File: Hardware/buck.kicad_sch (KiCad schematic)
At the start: 30 parts, among them Q301 SSM3K15AMFV,L3F, U301 SiC437AED-T1

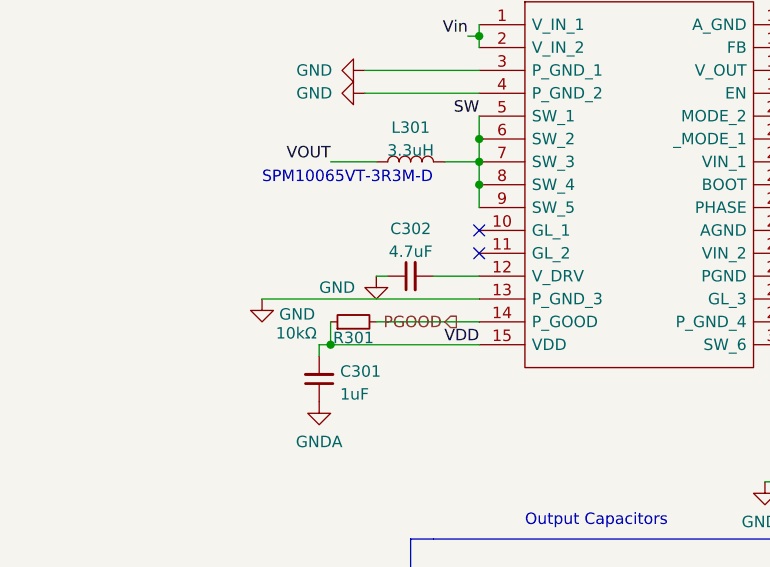
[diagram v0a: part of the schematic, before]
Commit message: prod files after final final change
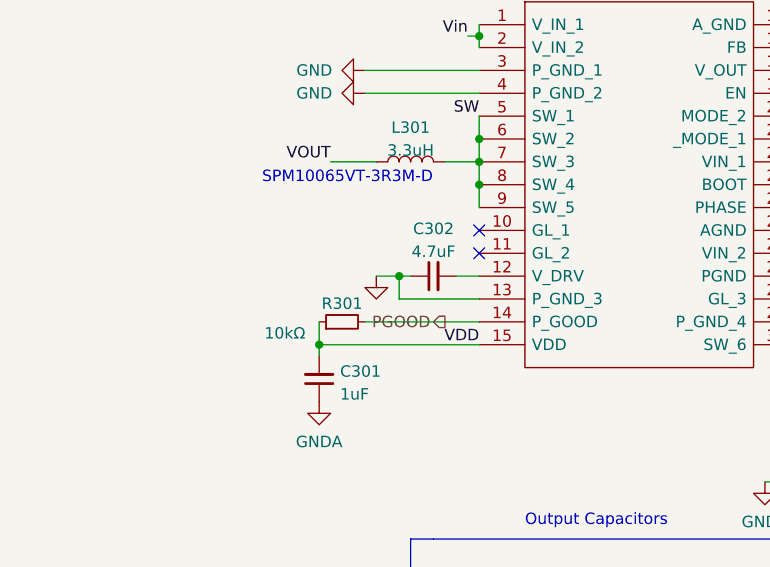
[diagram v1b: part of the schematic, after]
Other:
- moved on the sheet: C302, R301
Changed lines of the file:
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@@
 	)
 	(junction
-		(at 194.31 58.42)
+		(at 66.04 99.06)
 		(diameter 0)
 		(color 0 0 0 0)
 	)
 	(junction
-		(at 58.42 106.68)
+		(at 194.31 58.42)
 		(diameter 0)
 		(color 0 0 0 0)
@@
 	)
 	(junction
+		(at 57.15 106.68)
+		(diameter 0)
+		(color 0 0 0 0)
+	)
+	(junction
 		(at 208.28 77.47)
 		(diameter 0)
@@
 		)
 	)
+	(wire
+		(pts
+			(xy 66.04 99.06) (xy 66.04 101.6)
+		)
+		(stroke
+			(width 0)
+			(type default)
+		)
+	)
 	(polyline
 		(pts
@@
 	(wire
 		(pts
-			(xy 63.5 99.06) (xy 64.77 99.06)
-		)
-		(stroke
-			(width 0)
-			(type default)
-		)
-	)
-	(wire
-		(pts
-			(xy 58.42 104.14) (xy 58.42 106.68)
+			(xy 57.15 104.14) (xy 57.15 106.68)
 		)
 		(stroke
@@
 	(wire
 		(pts
-			(xy 86.36 140.97) (xy 91.44 140.97)
+			(xy 57.15 106.68) (xy 74.93 106.68)
 		)
 		(stroke
@@
 	(wire
 		(pts
-			(xy 58.42 106.68) (xy 57.15 106.68)
+			(xy 86.36 140.97) (xy 91.44 140.97)
 		)
 		(stroke
@@
 	(wire
 		(pts
-			(xy 63.5 104.14) (xy 74.93 104.14)
+			(xy 62.23 104.14) (xy 74.93 104.14)
 		)
 		(stroke
@@
 	(wire
 		(pts
+			(xy 66.04 101.6) (xy 74.93 101.6)
+		)
+		(stroke
+			(width 0)
+			(type default)
+		)
+	)
+	(wire
+		(pts
 			(xy 74.93 83.82) (xy 74.93 86.36)
 		)
@@
 	(wire
 		(pts
-			(xy 50.8 101.6) (xy 74.93 101.6)
+			(xy 63.5 99.06) (xy 66.04 99.06)
 		)
 		(stroke
@@
 	(wire
 		(pts
-			(xy 69.85 99.06) (xy 74.93 99.06)
+			(xy 72.39 99.06) (xy 74.93 99.06)
+		)
+		(stroke
+			(width 0)
+			(type default)
+		)
+	)
+	(wire
+		(pts
+			(xy 66.04 99.06) (xy 67.31 99.06)
 		)
 		(stroke
@@
 	(wire
 		(pts
-			(xy 58.42 106.68) (xy 74.93 106.68)
-		)
-		(stroke
-			(width 0)
-			(type default)
-		)
-	)
-	(wire
-		(pts
 			(xy 124.46 69.85) (xy 134.62 69.85)
 		)
@@
 	(hierarchical_label "PGOOD"
 		(shape output)
-		(at 72.39 104.14 180)
+		(at 71.12 104.14 180)
 		(effects
 			(font
@@
 	(symbol
 		(lib_id "Device:C_Small")
-		(at 67.31 99.06 90)
+		(at 69.85 99.06 90)
 		(unit 1)
 		(exclude_from_sim no)
@@
 		(fields_autoplaced yes)
 		(property "Reference" "C302"
-			(at 67.3163 93.7981 90)
+			(at 69.8563 93.7981 90)
 			(effects
 				(font
@@
 		)
 		(property "Value" "4.7uF"
-			(at 67.3163 96.335 90)
+			(at 69.8563 96.335 90)
 			(effects
 				(font
@@
 		)
 		(property "Footprint" "Capacitor_SMD:C_0402_1005Metric"
-			(at 67.31 99.06 0)
+			(at 69.85 99.06 0)
 			(effects
 				(font
@@
 		)
 		(property "Datasheet" "~"
-			(at 67.31 99.06 0)
+			(at 69.85 99.06 0)
 			(effects
 				(font
@@
 		)
 		(property "Description" ""
-			(at 67.31 99.06 0)
+			(at 69.85 99.06 0)
 			(effects
 				(font
@@
 	(symbol
 		(lib_id "Device:R_Small")
-		(at 60.96 104.14 90)
+		(at 59.69 104.14 90)
 		(unit 1)
 		(exclude_from_sim no)
@@
 		(dnp no)
 		(property "Reference" "R301"
-			(at 60.96 105.918 90)
+			(at 59.69 102.108 90)
 			(effects
 				(font
@@
 		)
 		(property "Value" "10kΩ"
-			(at 54.61 105.4069 90)
+			(at 53.34 105.4069 90)
 			(effects
 				(font
@@
 		)
 		(property "Footprint" "Resistor_SMD:R_0402_1005Metric"
-			(at 60.96 104.14 0)
+			(at 59.69 104.14 0)
 			(effects
 				(font
@@
 		)
 		(property "Datasheet" "~"
-			(at 60.96 104.14 0)
+			(at 59.69 104.14 0)
 			(effects
 				(font
@@
 		)
 		(property "Description" ""
-			(at 60.96 104.14 0)
+			(at 59.69 104.14 0)
 			(effects
 				(font
@@
 				)
 				(justify left)
+				(hide yes)
 			)
 		)
@@
 					(unit 1)
 				)
-			)
-		)
-	)
-	(symbol
-		(lib_id "power:GND")
-		(at 50.8 101.6 0)
-		(unit 1)
-		(exclude_from_sim no)
-		(in_bom yes)
-		(on_board yes)
-		(dnp no)
-		(fields_autoplaced yes)
-		(property "Reference" "#PWR0301"
-			(at 50.8 107.95 0)
-			(effects
-				(font
-					(size 1.27 1.27)
-				)
-				(hide yes)
-			)
-		)
-		(property "Value" "GND"
-			(at 52.705 103.3038 0)
-			(effects
-				(font
-					(size 1.27 1.27)
-				)
-				(justify left)
-			)
-		)
-		(property "Footprint" ""
-			(at 50.8 101.6 0)
-			(effects
-				(font
-					(size 1.27 1.27)
-				)
-				(hide yes)
-			)
-		)
-		(property "Datasheet" ""
-			(at 50.8 101.6 0)
-			(effects
-				(font
-					(size 1.27 1.27)
-				)
-				(hide yes)
-			)
-		)
-		(property "Description" ""
-			(at 50.8 101.6 0)
-			(effects
-				(font
-					(size 1.27 1.27)
-				)
-				(hide yes)
-			)
-		)
-		(pin "1"
-		)
-		(instances
-			(project "Heimdall"
-				(path "/7db990e4-92e1-4f99-b4d2-435bbec1ba83/4df4c1d6-182a-4df8-9cbb-8b8cf0f2cf46"
-					(reference "#PWR0301")
-					(unit 1)
-				)
